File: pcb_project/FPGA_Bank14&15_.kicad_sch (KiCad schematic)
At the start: 30 parts, among them IC3 IS61WV204816BLL-10TLI, U1 XC7A100T-FTG256, U9 MT25QL128ABA1ESE-0SIT

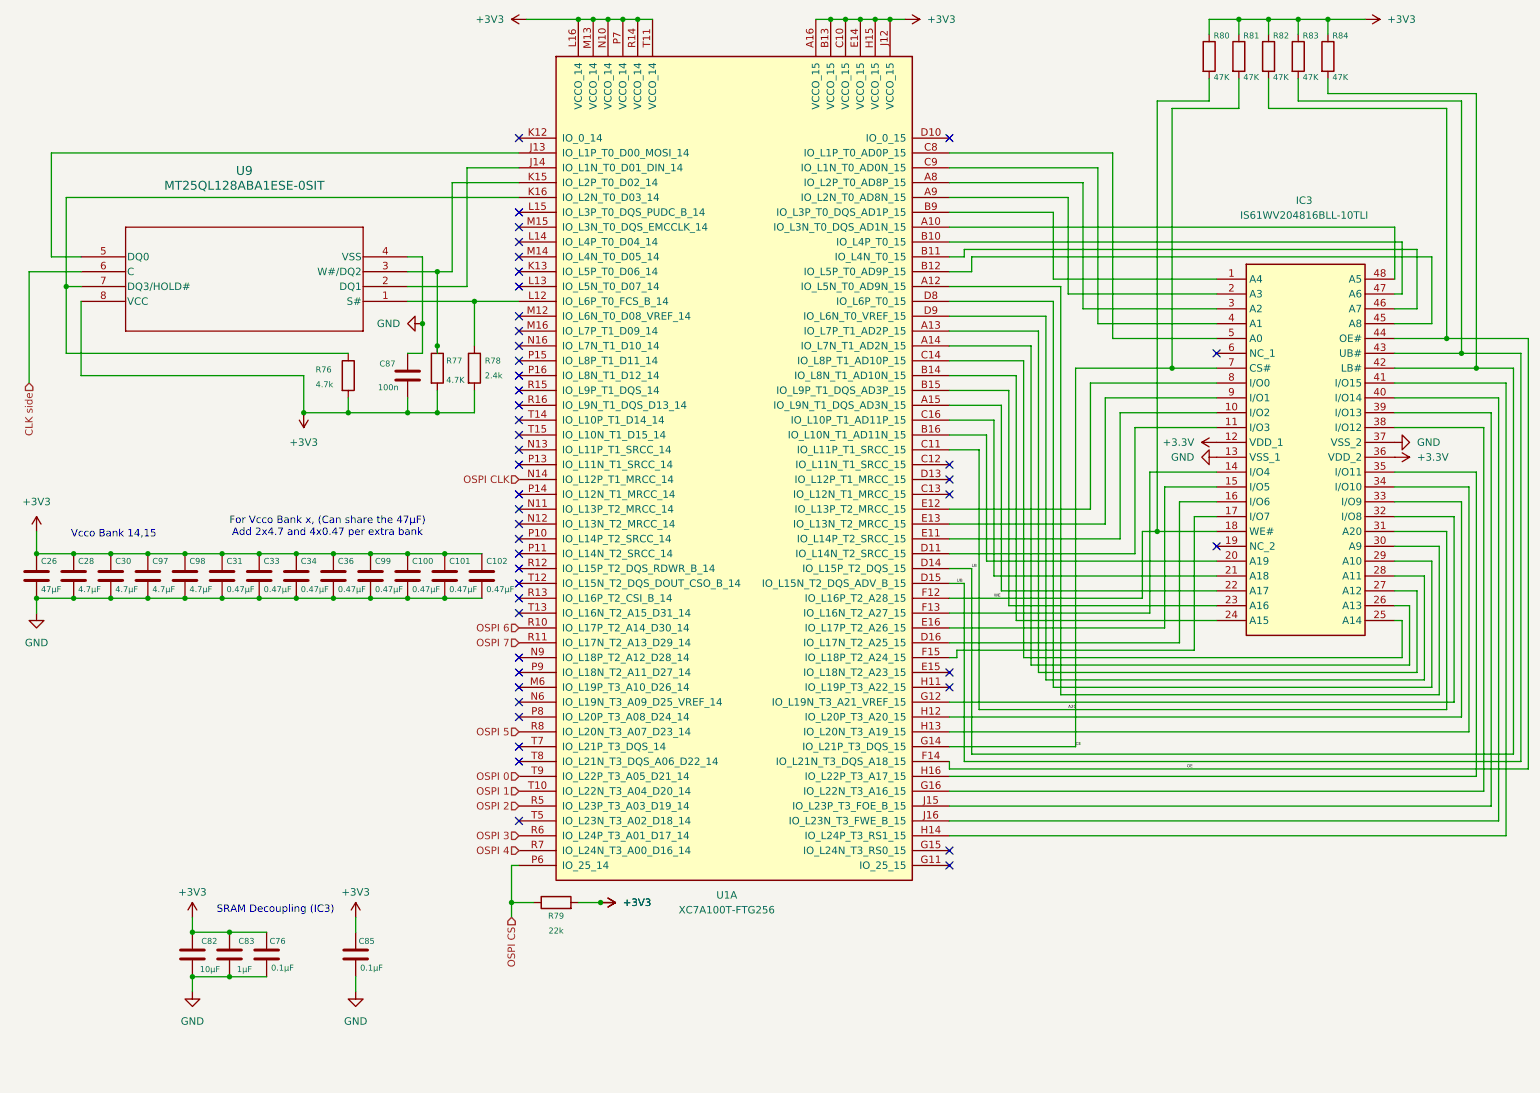
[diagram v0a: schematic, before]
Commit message: FPGA decoupler
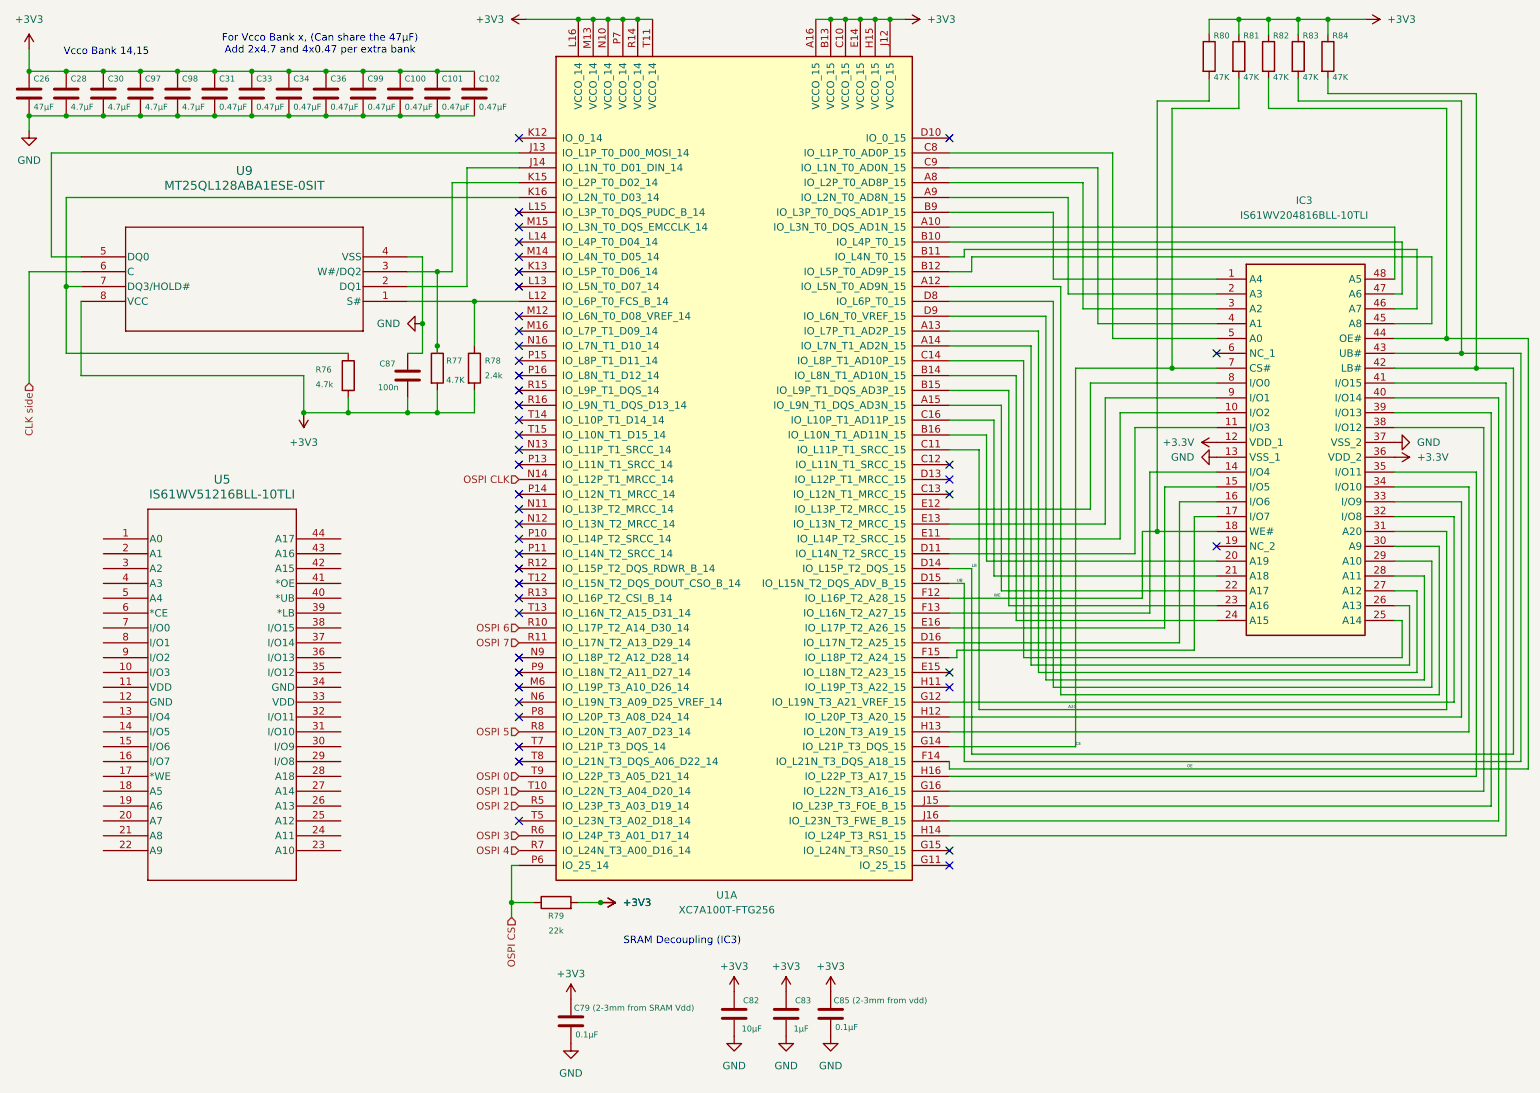
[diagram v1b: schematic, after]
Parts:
- removed C76: 0.1µF, Capacitor_SMD:C_0603_1608Metric_Pad1.08x0.95mm_HandSolder, symbol Device:C
- added C79 (2-3mm from SRAM Vdd): 0.1µF, Capacitor_SMD:C_0603_1608Metric_Pad1.08x0.95mm_HandSolder, symbol Device:C
- added U5: IS61WV51216BLL-10TLI, TSOP-2_44L_400MIL_ISI, symbol Is61Wv51216BLL:IS61WV51216BLL-10TLI
- C85 (2-3mm from vdd): renamed from C85
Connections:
- net +3V3: now also C79 (2-3mm from SRAM Vdd).1
- net GND: now also C79 (2-3mm from SRAM Vdd).2
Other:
- moved on the sheet: C100, C101, C102, C26, C28, C30, C31, C33, C34, C36, C82, C83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
